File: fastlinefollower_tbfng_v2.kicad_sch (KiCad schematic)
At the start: 12 parts, among them J1 IR_conn, J2 Motor1, J3 Motor2, SW1 Run, SW2 Calibrate, SW3 SW_SPST, U1 TB6612FNG_Module, U2 LM7805_TO220

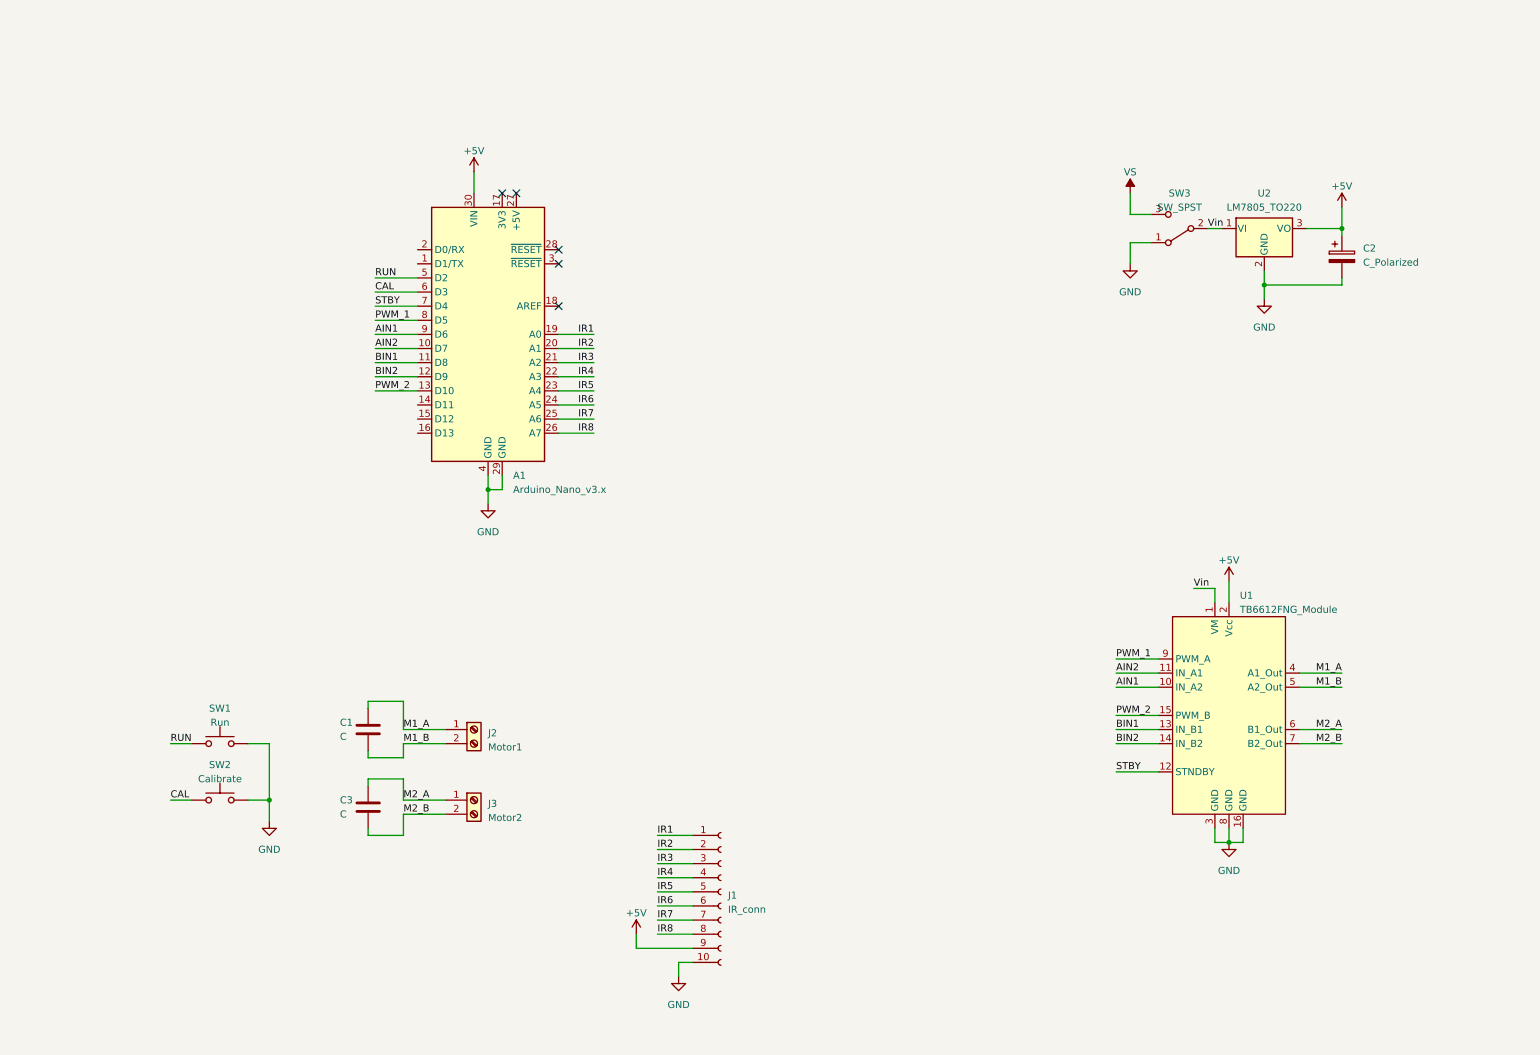
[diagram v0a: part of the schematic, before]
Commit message: final twicks
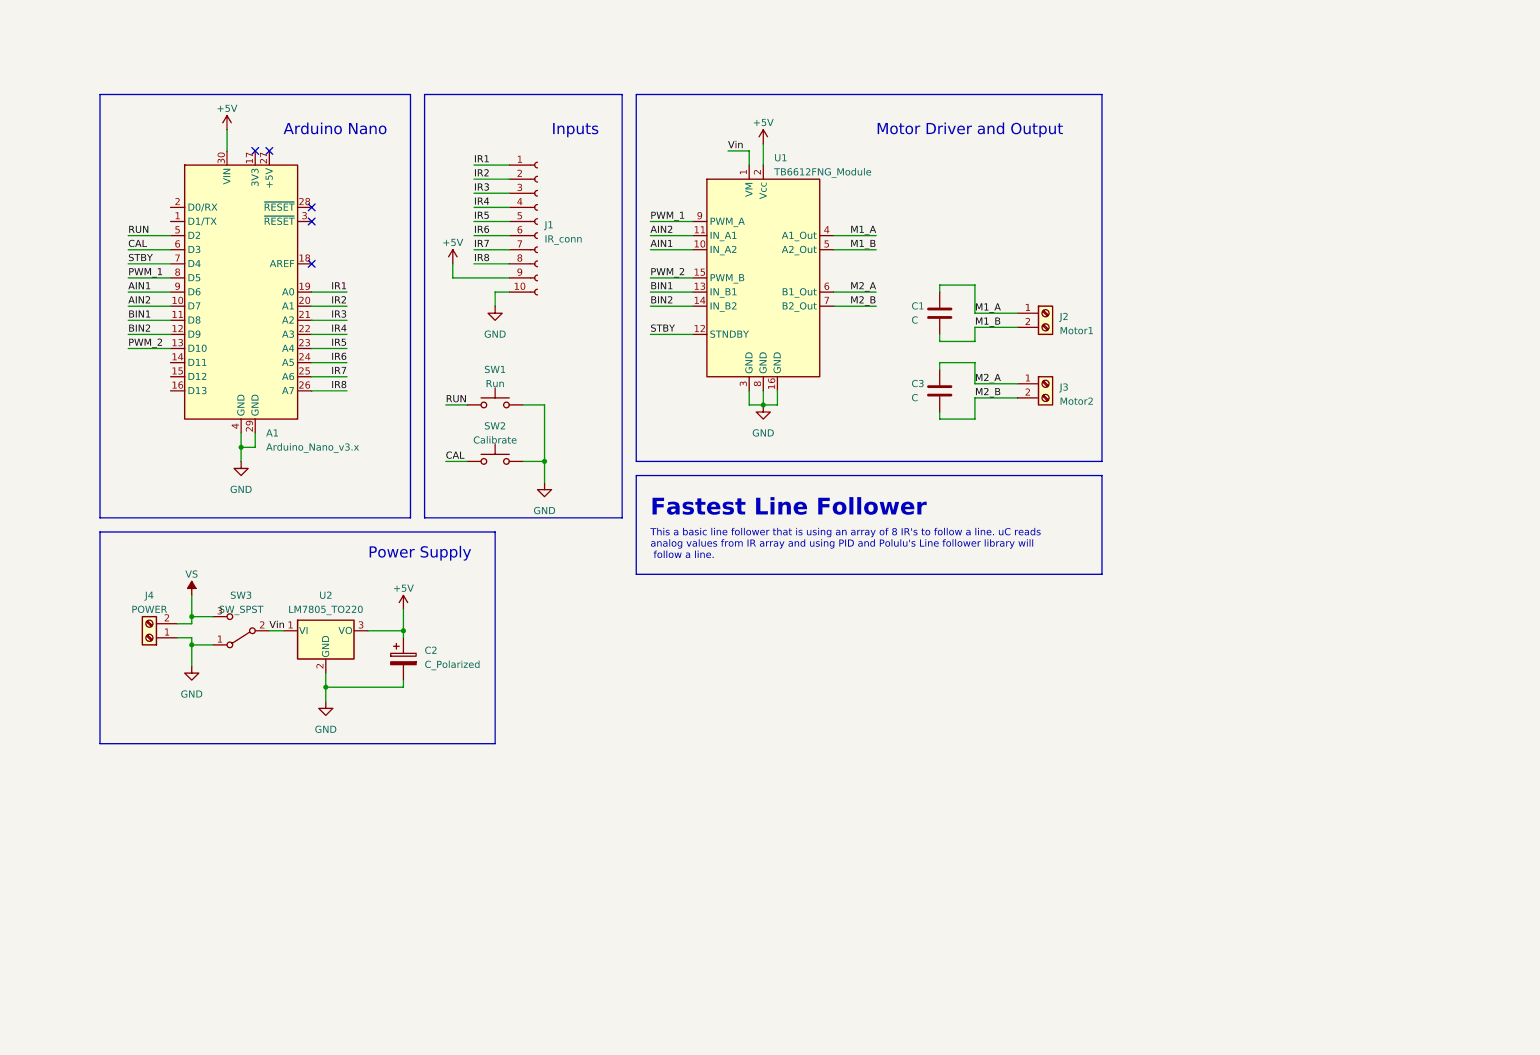
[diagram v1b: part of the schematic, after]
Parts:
- added J4: POWER, TerminalBlock:TerminalBlock_bornier-2_P5.08mm, symbol Connector:Screw_Terminal_01x02
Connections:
- net GND: now also J4.1 (Pin_1)
- net VS: now also J4.2 (Pin_2)
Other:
- note added: "Arduino Nano"
- note added: "Fastest Line Follower"
- note added: "Inputs"
- note added: "Motor Driver and Output"
- note added: "Power Supply"
- note added: "This a basic line follower that is using an array of 8 IR's to follow a line. uC reads analog values from IR array and using PID and Polulu's Line follower library will follow a line."
- company: (none) -> DRAIC
- title: (none) -> Fastest Line Follower
- moved on the sheet: A1, C1, C2, C3, J1, J2, J3, SW1, SW2, SW3, U1, U2
